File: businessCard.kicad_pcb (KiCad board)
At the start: 2 copper layers, 88.6 x 50.6 mm, 33 parts

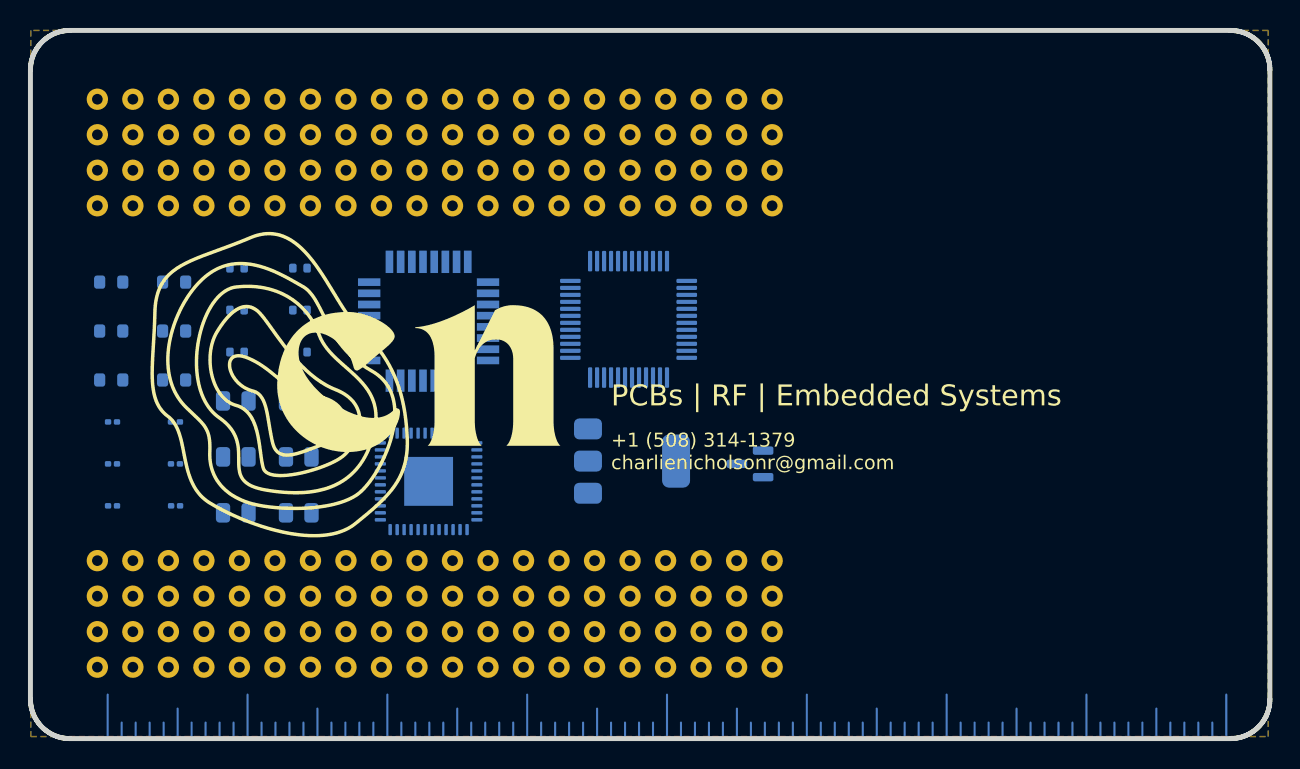
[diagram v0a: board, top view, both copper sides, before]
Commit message: Added some stuff
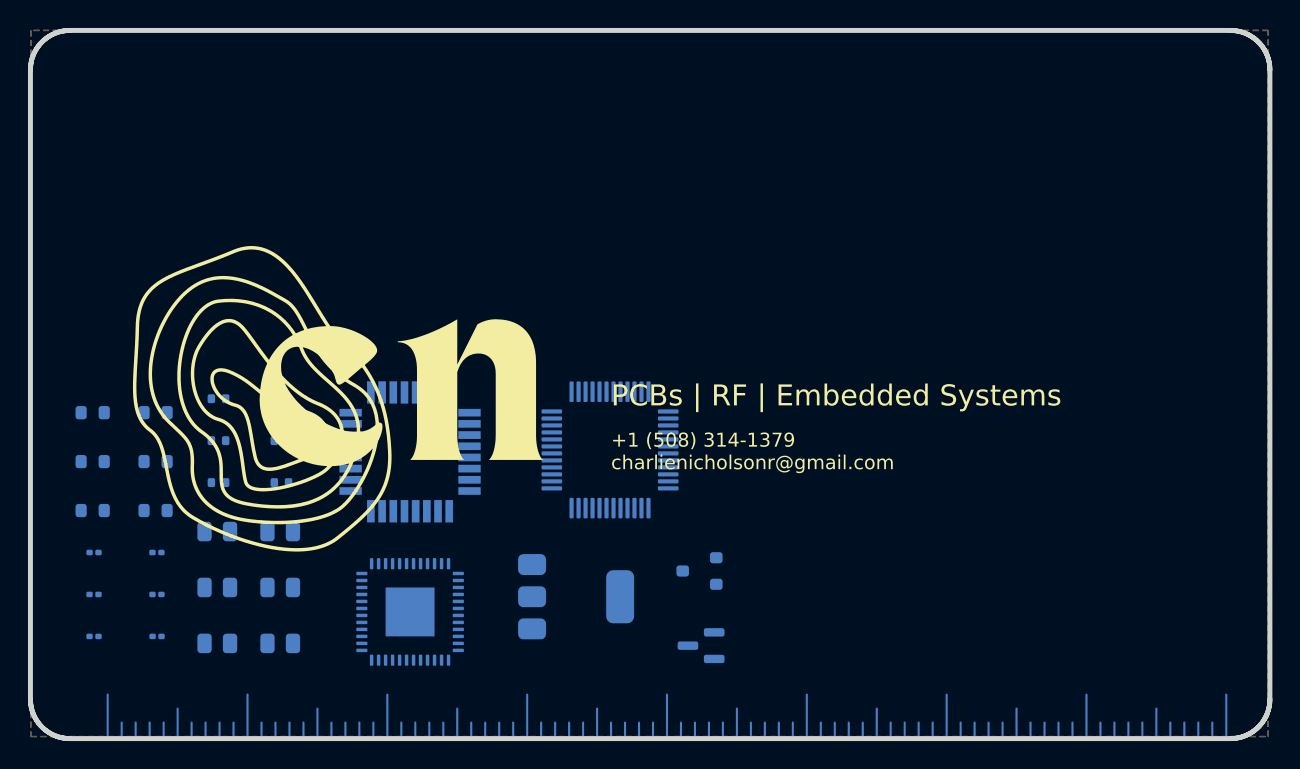
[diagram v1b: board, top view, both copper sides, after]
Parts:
- removed REF** (x2): Perf_Board, Connector_PinHeader_2.54mm:Perf_Board
- added SC-59: SC-59, Package_TO_SOT_SMD:SC-59, B.Cu at (147.8, 78.7)
- moved SOT-23 13.5 mm to (147.9, 84.0)
- moved SOT-223 10.5 mm to (139.0, 80.5)
- moved 0201 9.43 mm to (109.0, 83.3)
- moved 0201 9.43 mm to (104.5, 83.3)
- moved 0201 9.43 mm to (104.5, 77.3)
- moved 0201 9.43 mm to (109.0, 80.3)
- moved 0201 9.43 mm to (109.0, 77.3)
- moved 0201 9.43 mm to (104.5, 80.3)
- moved 0402 9.43 mm to (113.4, 66.3)
- moved 0402 9.43 mm to (113.4, 72.3)
- moved 0402 9.43 mm to (113.4, 69.3)
- moved 0402 9.43 mm to (117.9, 69.3)
- moved 0402 9.43 mm to (117.9, 72.3)
- moved 0402 9.43 mm to (117.9, 66.3)
- moved 0603 9.43 mm to (108.9, 67.3)
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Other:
- board text added: "Calculations: V_{drop} = IR P_{loss} = RI^{2}"
- board text added: "Conversions: 1 in = 25.4 mm 1 mm = 0.04 in 1 kg = 2.205 lbs 1 lb = 453.59 g Fahrenheit = (9/5 X deg C) + 32 Celsius = 5/9 X (deg F - 32)"
- board text removed: "Mini perf board"
